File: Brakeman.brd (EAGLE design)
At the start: 25 x 29.5 mm, 9 parts

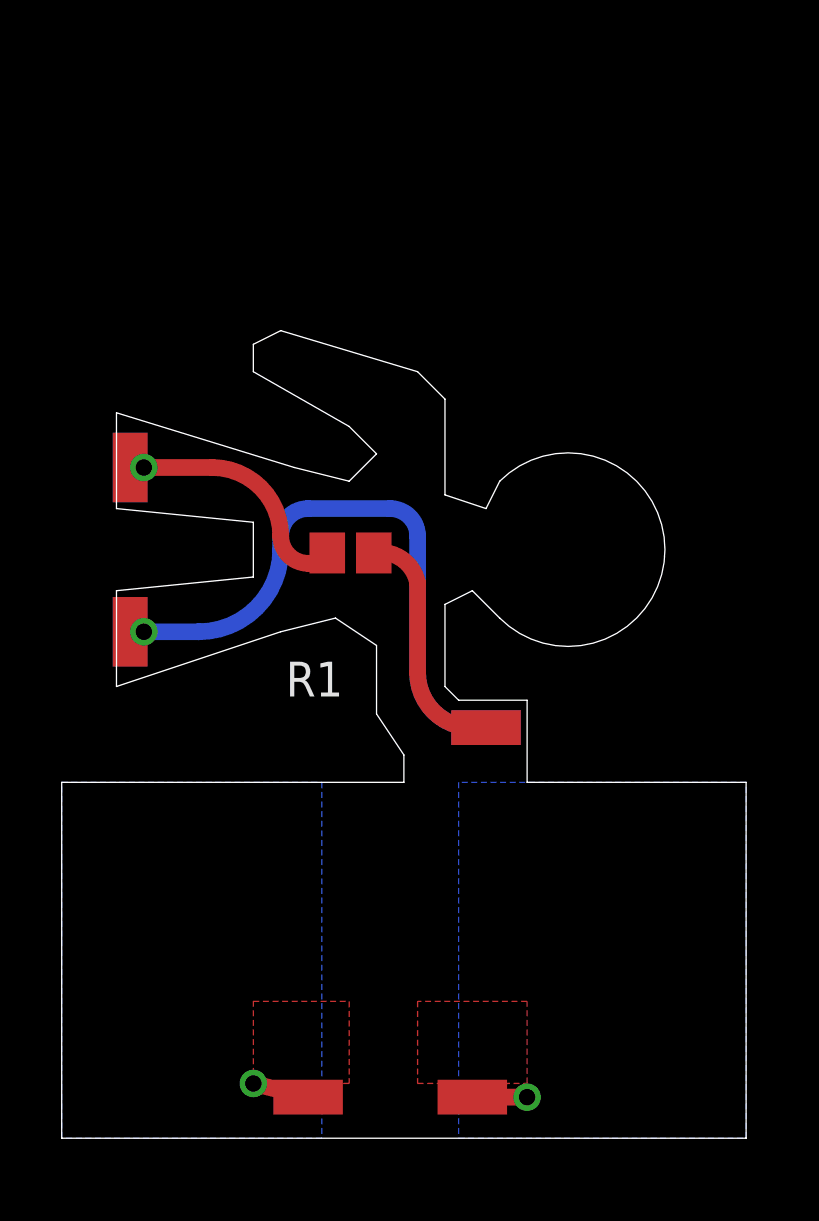
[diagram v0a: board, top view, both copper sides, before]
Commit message: 1.2
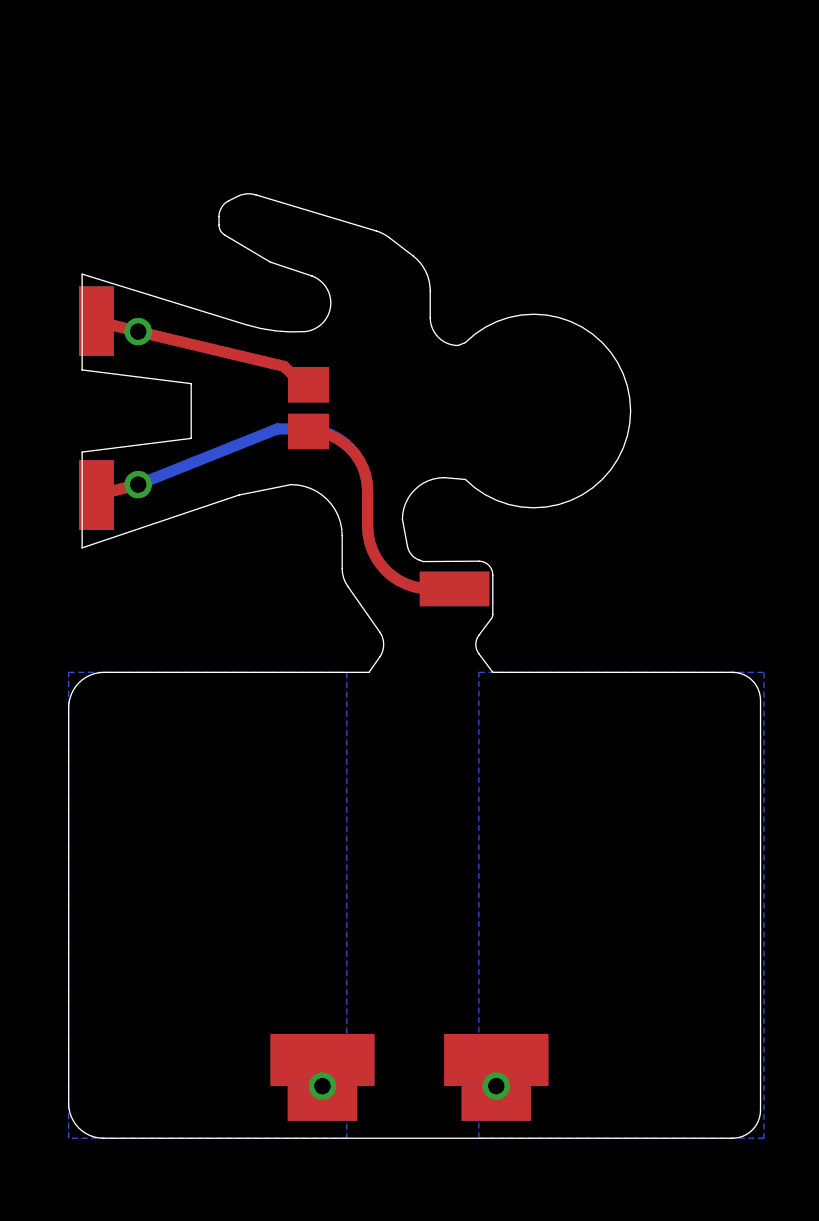
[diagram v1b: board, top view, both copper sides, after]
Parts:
- removed PAD3, PAD4, PAD5, PAD6, PAD7, PAD8: (no value), wirepad:SMD1.27-2.54
- added PAD10, PAD11, PAD12, PAD14, PAD20, PAD21, PAD23, PAD24: (no value), wirepad:SMD1.27-2.54
- moved PAD1 15.0 mm to (9.53, 1.27), flipped to the bottom, turned to 90 degrees
- moved PAD2 13.7 mm to (15.9, 1.27)
- moved R1 5.51 mm to (9.02, 26.7), turned to 90 degrees
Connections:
- removed net N$2: PAD1.1, R1.1
- new net N$3: PAD14.1, R1.1
- net N: now also PAD20.1, PAD21.1, PAD23.1, PAD24.1; no longer PAD4.1, PAD6.1, PAD8.1
- net S: now also PAD1.1, PAD10.1, PAD11.1, PAD12.1; no longer PAD3.1, PAD5.1, PAD7.1
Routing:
- net N$2: track 8.55 -> 0.00 mm
- net N$3: track 0.00 -> 8.48 mm
- net N: track 23.5 -> 19.5 mm
- removed copper zone on layer 1, net N
- removed copper zone on layer 1, net S
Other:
- board size 25 x 29.5 mm -> 25.3 x 34.5 mm
- board text added: "2012.04"
- board text added: "Add"
- board text added: "DCC"
- board text added: "here"
- board text added: "weight"
- board text removed: "2012.01"

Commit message: 1.3
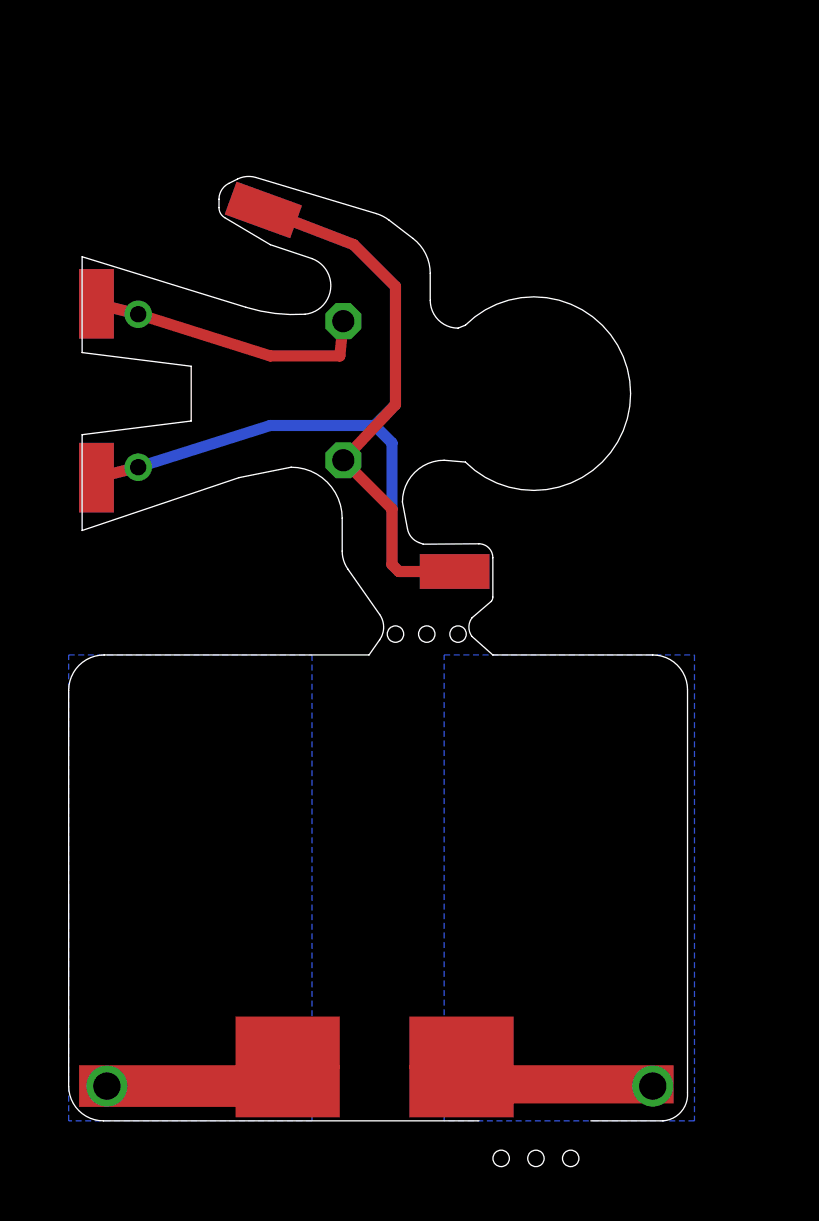
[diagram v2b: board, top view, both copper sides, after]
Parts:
- removed PAD1, PAD10, PAD11, PAD12, PAD14, PAD2, PAD20, PAD21, PAD23, PAD24: (no value), wirepad:SMD1.27-2.54
- added PADL1, PADL2, PADN2, PADN3, PADN4, PADN6, PADS2, PADS4: (no value), wirepad:SMD1.27-2.54
- R1: value (none) -> 1k0; device resistor:R0805 -> resistor:0204/5
- moved R1 1.42 mm to (10.3, 27.3), flipped to the bottom
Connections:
- removed net N$3: PAD14.1, R1.1
- new net LIMITED: PADL1.1, PADL2.1, R1.1
- net N: now also PADN2.1, PADN3.1, PADN4.1, PADN6.1; no longer PAD2.1, PAD20.1, PAD21.1, PAD23.1, PAD24.1
- net S: now also PADS2.1, PADS4.1; no longer PAD1.1, PAD10.1, PAD11.1, PAD12.1
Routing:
- net LIMITED: track 0.00 -> 19.7 mm
- net N: track 19.5 -> 31.5 mm
- net N$3: track 8.48 -> 0.00 mm
- net S: track 11.0 -> 12.0 mm
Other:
- board size 25.3 x 34.5 mm -> 22.6 x 34.5 mm
- board text added: "2016.04"
- board text added: "DCC Flagman & Fusee"
- board text added: "Flagman"
- board text added: "www.SPCoast.com"
- board text removed: "2012.04"
- board text removed: "Brakeman"
- board text removed: "DCC Brakeman"

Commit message: 2.0
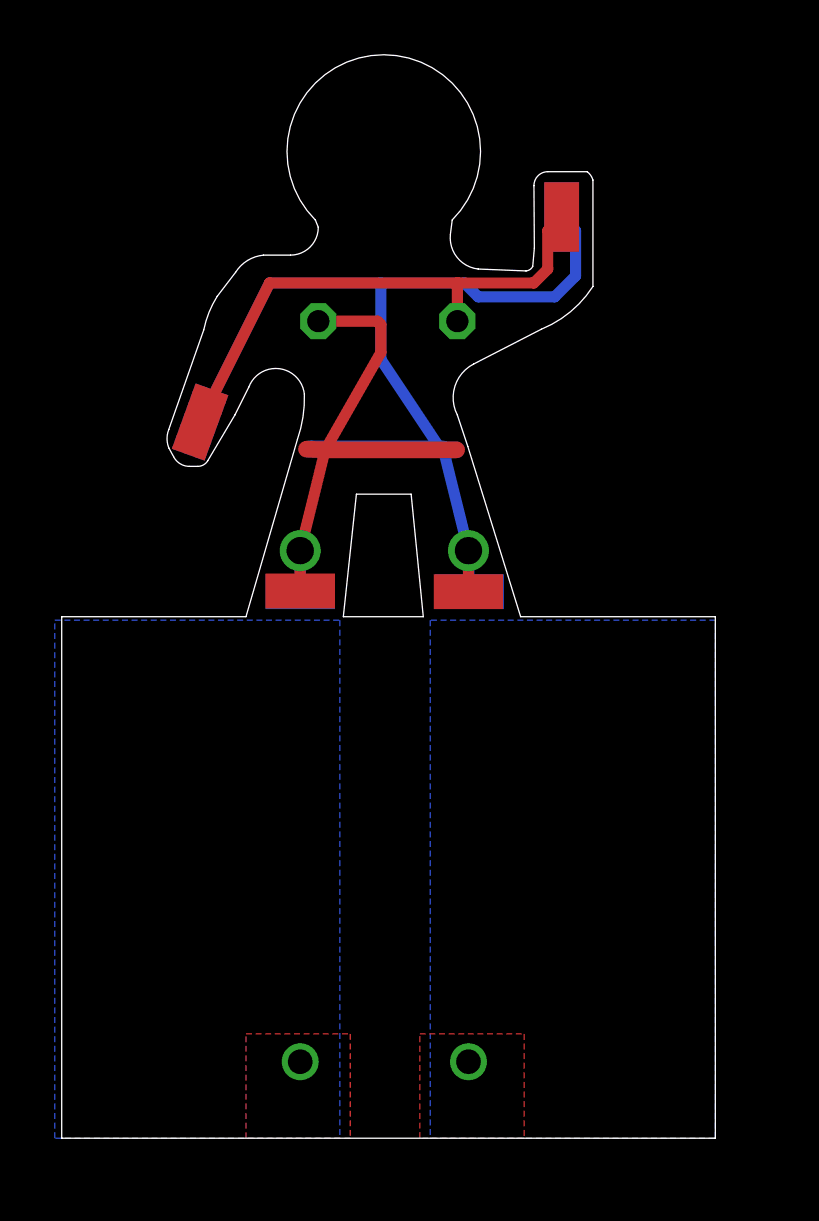
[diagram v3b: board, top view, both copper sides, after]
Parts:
- removed PADN2, PADN3, PADN4, PADN6, PADS2, PADS4: (no value), wirepad:SMD1.27-2.54
- added PADNA, PADNA2, PADNF, PADNF2, PADSF, PADSF2: (no value), wirepad:SMD1.27-2.54
- moved PADL2 10.9 mm to (18.3, 33.7), turned to 0 degrees
- moved PADL1 10.8 mm to (5.05, 26.2), turned to 160 degrees
- moved R1 3.02 mm to (11.9, 29.8), turned to 0 degrees
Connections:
- net N: now also PADNA.1, PADNA2.1, PADNF.1, PADNF2.1; no longer PADN2.1, PADN3.1, PADN4.1, PADN6.1
- net S: now also PADSF.1, PADSF2.1; no longer PADS2.1, PADS4.1
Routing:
- net S: track 12.0 -> 19.7 mm
- net N: track 31.5 -> 38.9 mm
- added copper zone on layer 1, net N
- added copper zone on layer 1, net S
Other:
- board size 22.6 x 34.5 mm -> 23.9 x 39.6 mm
- board text added: "DCC Flagman"
- board text removed: "DCC Flagman & Fusee"
